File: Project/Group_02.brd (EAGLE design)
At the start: 29 parts, among them J1 POWER_JACKPTH_LOCK, U1 +12v

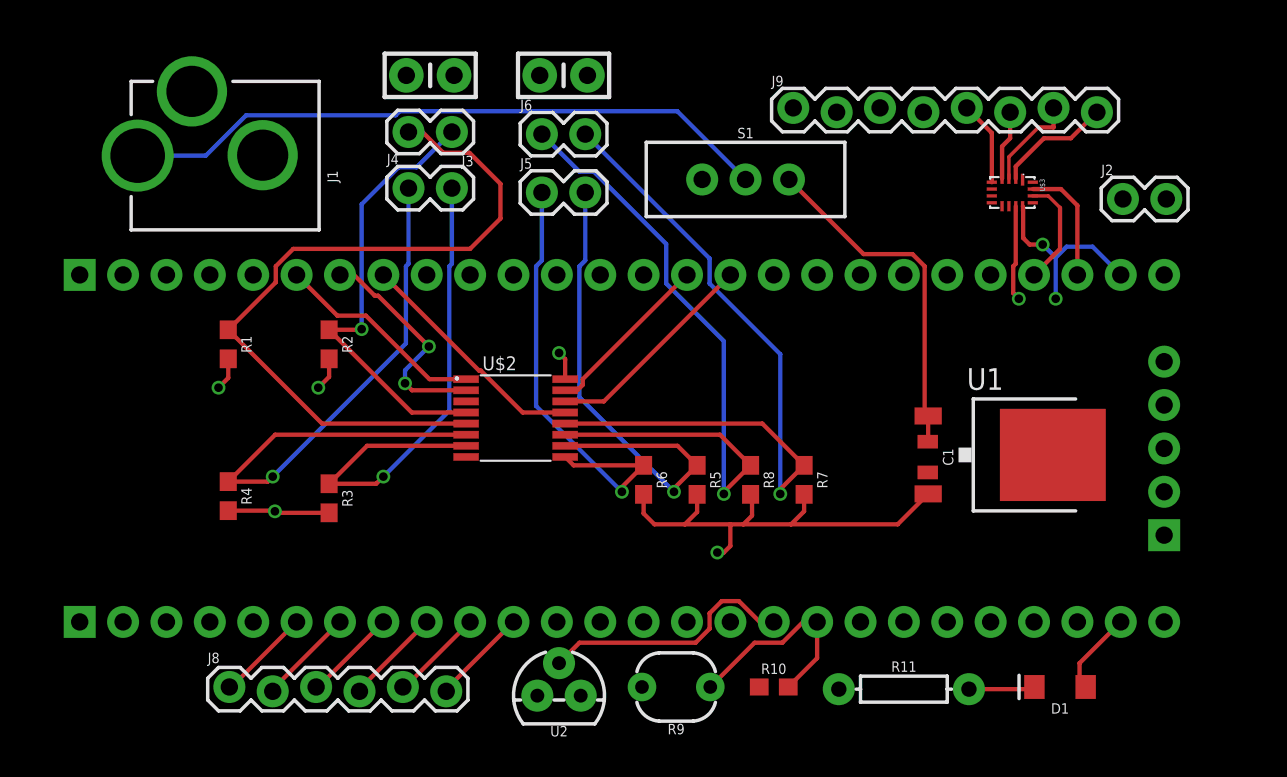
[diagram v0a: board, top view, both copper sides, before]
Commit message: Piccole modifiche e spostamenti
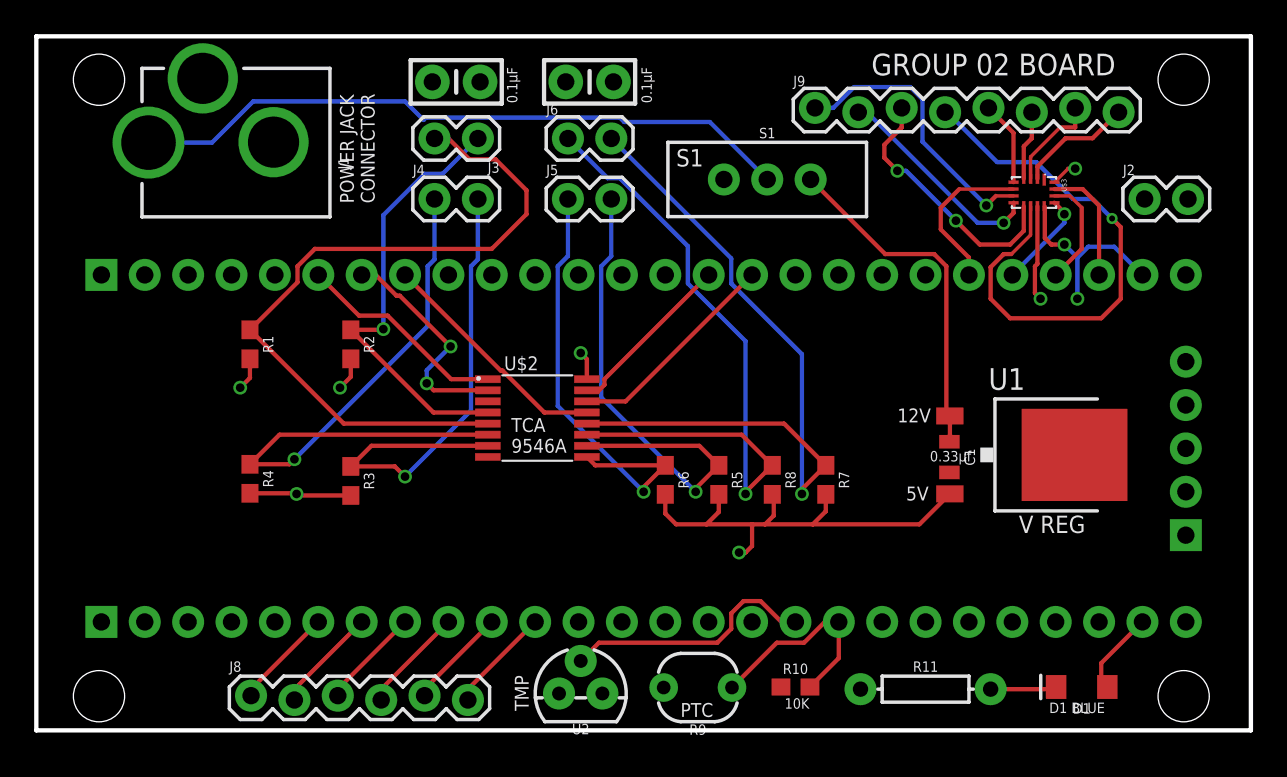
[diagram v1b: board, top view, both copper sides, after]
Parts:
- moved J4 1.65 mm to (23.3, 31.1)
- moved R3 1.63 mm to (18.4, 14.6)
- moved R4 1.63 mm to (12.5, 14.7)
- moved C2 1.57 mm to (24.6, 38.0)
- moved C3 1.57 mm to (32.4, 38.0)
- moved J5 1.57 mm to (31.1, 31.1)
- moved J3 1.57 mm to (25.9, 34.7)
- moved J6 1.55 mm to (31.1, 34.7)
- moved J8 1.37 mm to (12.6, 2.03)
- moved U2 1.28 mm to (31.9, 2.16)
- moved R9 1.27 mm to (38.7, 2.51)
- moved J2 1.27 mm to (64.9, 31.1)
- moved J9 1.27 mm to (45.6, 36.3)
- moved R10 1.27 mm to (44.5, 2.54)
- moved R11 1.27 mm to (52.1, 2.41)
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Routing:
- net N$14: track 0.13 -> 32.5 mm, vias 0 -> 1
- net N$17: track 0.00 -> 16.7 mm, vias 0 -> 1
- net N$15: track 0.00 -> 15.4 mm, vias 0 -> 2
- net N$16: track 0.00 -> 12.6 mm, vias 0 -> 1
- net MUX_OUT: track 0.00 -> 9.33 mm
- net MUX_A2: track 0.00 -> 5.73 mm, vias 0 -> 1
- net I2C_SDA_1: track 38.0 -> 36.0 mm
- net 5V: track 44.3 -> 45.8 mm, vias 6 -> 7
- net N$1: track 38.3 -> 39.2 mm
- net I2C_SCL_1: track 30.8 -> 30.0 mm
- net N$7: track 5.69 -> 6.20 mm
- net N$3: track 5.69 -> 6.20 mm
- net N$5: track 5.69 -> 6.20 mm
- added copper zone on layer 16, net 5V
- added copper zone on layer 1, net GND
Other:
- board outline added: 71.1 x 40.6 mm
- board text added: "0.1μF"
- board text added: "0.33μf"
- board text added: "10K"
- board text added: "12V"
- board text added: "5V"
- board text added: "CY8CKIT059-TARGET"
- board text added: "D1 BLUE"
- board text added: "GND"
- board text added: "GROUP 02 BOARD"
- board text added: "MUX PINS"
- board text added: "POWER JACK CONNECTOR"
- board text added: "PTC"
- board text added: "S1"
- board text added: "TCA 9546A"
- board text added: "TMP"
- board text added: "V REG"
